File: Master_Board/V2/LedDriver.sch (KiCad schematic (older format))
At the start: 2 parts

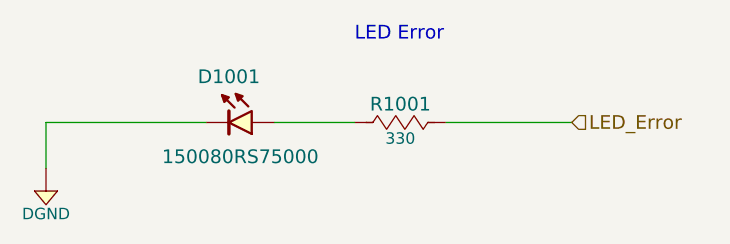
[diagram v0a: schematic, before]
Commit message: Done placing parts on PCB
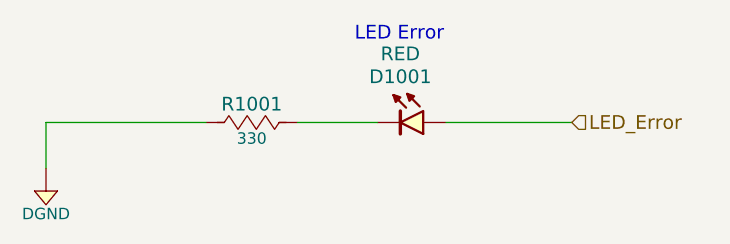
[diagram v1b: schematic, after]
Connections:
- net DGND: now also R1001.1; no longer D1001.1 (Cathode)
- net LED_Error: now also D1001.2 (Anode); no longer R1001.2
- new net: D1001.1 (Cathode), R1001.2
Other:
- moved on the sheet: D1001, R1001
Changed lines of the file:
@@
 L 150080RS75000 D1001
 U 1 1 594D45D6
-P 5350 3700
-F 0 "D1001" H 5350 3500 60  0000 C CNN
-F 1 "150080RS75000" H 5300 3850 60  0000 C CNN
-F 2 "Diodes:LED_0805_RED" H 5360 2620 60  0001 C CNN
-F 3 "http://katalog.we-online.de/led/datasheet/150080RS75000.pdf" H 5360 2520 60  0001 C CNN
-F 4 "Digikey" H 5360 3120 60  0001 C CNN "Supplier"
-F 5 "732-4984-1-ND" H 5360 3020 60  0001 C CNN "Supplier Part Number"
-F 6 "Wurth Electronics Inc." H 5360 2920 60  0001 C CNN "Manufacturer"
-F 7 "150080RS75000" H 5360 2820 60  0001 C CNN "Manufacturer Part Number"
-F 8 "LED RED CLEAR 0805 SMD" H 5360 2720 60  0001 C CNN "Description"
-F 9 "RED" H 5350 3400 60  0001 C CNN "Color"
-F 10 "2V" H 5350 3300 60  0001 C CNN "Voltage - Forward (Vf) (Typ)"
-	1    5350 3700
+P 6100 3700
+F 0 "D1001" H 6100 3500 60  0000 C CNN
+F 1 "150080RS75000" H 6050 3850 60  0001 C CNN
+F 2 "Diodes:LED_0805_RED" H 6110 2620 60  0001 C CNN
+F 3 "http://katalog.we-online.de/led/datasheet/150080RS75000.pdf" H 6110 2520 60  0001 C CNN
+F 4 "Digikey" H 6110 3120 60  0001 C CNN "Supplier"
+F 5 "732-4984-1-ND" H 6110 3020 60  0001 C CNN "Supplier Part Number"
+F 6 "Wurth Electronics Inc." H 6110 2920 60  0001 C CNN "Manufacturer"
+F 7 "150080RS75000" H 6110 2820 60  0001 C CNN "Manufacturer Part Number"
+F 8 "LED RED CLEAR 0805 SMD" H 6110 2720 60  0001 C CNN "Description"
+F 9 "RED" H 6100 3400 60  0000 C CNN "Color"
+F 10 "2V" H 6100 3300 60  0001 C CNN "Voltage - Forward (Vf) (Typ)"
+	1    6100 3700
 	-1   0    0    1
 $EndComp
@@
 L RC0805JR-07330RL R1001
 U 1 1 594D472A
-P 6100 3700
-F 0 "R1001" H 6100 3780 60  0000 C CNN
-F 1 "RC0805JR-07330RL" H 6100 3400 50  0001 C CNN
-F 2 "Resistors:R0805" H 6100 2800 30  0001 C CNN
-F 3 "http://www.yageo.com/documents/recent/PYu-RC_Group_51_RoHS_L_7.pdf" H 6100 2750 30  0001 C CNN
-F 4 "Digikey" H 6100 3300 60  0001 C CNN "Supplier"
-F 5 "311-330ARCT-ND" H 6100 3200 60  0001 C CNN "Supplier Part Number"
-F 6 "Yageo" H 6100 3100 60  0001 C CNN "Manufacturer"
-F 7 "RC0805JR-07330RL" H 6100 3000 60  0001 C CNN "Manufacturer Part Number"
-F 8 "RES SMD 330 OHM 5% 1/8W 0805" H 6100 2900 60  0001 C CNN "Description"
-F 9 "330" H 6100 3630 50  0000 C CNN "Resistance (Ohms)"
-F 10 "±5%" H 6510 3620 50  0001 C CNN "Tolerance (%)"
-F 11 "1/8W" H 6100 3560 50  0001 C CNN "Puissance (Watts)"
-	1    6100 3700
+P 5450 3700
+F 0 "R1001" H 5450 3780 60  0000 C CNN
+F 1 "RC0805JR-07330RL" H 5450 3400 50  0001 C CNN
+F 2 "Resistors:R0805" H 5450 2800 30  0001 C CNN
+F 3 "http://www.yageo.com/documents/recent/PYu-RC_Group_51_RoHS_L_7.pdf" H 5450 2750 30  0001 C CNN
+F 4 "Digikey" H 5450 3300 60  0001 C CNN "Supplier"
+F 5 "311-330ARCT-ND" H 5450 3200 60  0001 C CNN "Supplier Part Number"
+F 6 "Yageo" H 5450 3100 60  0001 C CNN "Manufacturer"
+F 7 "RC0805JR-07330RL" H 5450 3000 60  0001 C CNN "Manufacturer Part Number"
+F 8 "RES SMD 330 OHM 5% 1/8W 0805" H 5450 2900 60  0001 C CNN "Description"
+F 9 "330" H 5450 3630 50  0000 C CNN "Resistance (Ohms)"
+F 10 "±5%" H 5860 3620 50  0001 C CNN "Tolerance (%)"
+F 11 "1/8W" H 5450 3560 50  0001 C CNN "Puissance (Watts)"
+	1    5450 3700
 	1    0    0    -1
 $EndComp
 Wire Wire Line
-	5900 3700 5550 3700
+	5650 3700 6000 3700
 Text HLabel 6850 3700 2    60   Input ~ 0
 LED_Error
